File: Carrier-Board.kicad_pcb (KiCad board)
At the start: 2 copper layers, 92 x 96 mm, 5 parts, among them J1 CONN_3-6318491-6, J2 SI-51009-F, U1 MSATA-Socket, X1 PC104_PLUS

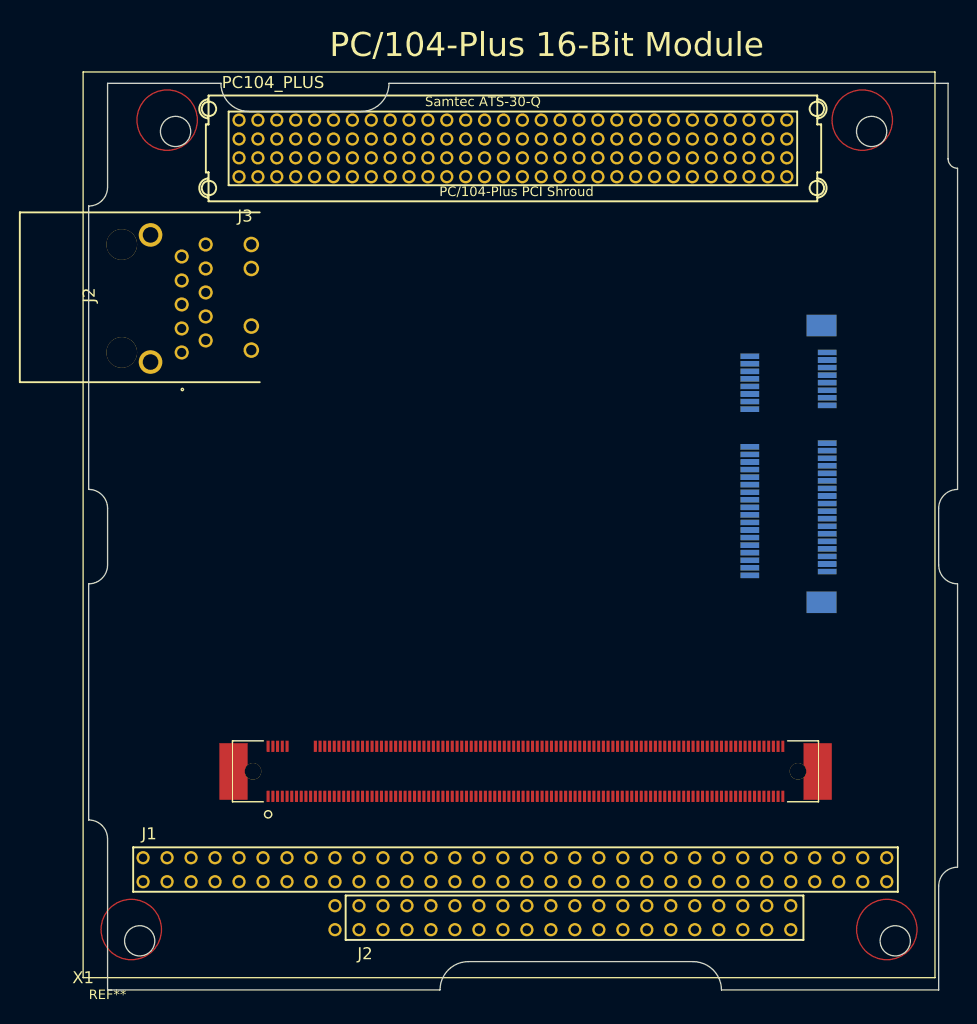
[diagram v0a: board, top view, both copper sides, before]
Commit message: Remove junk from pc104
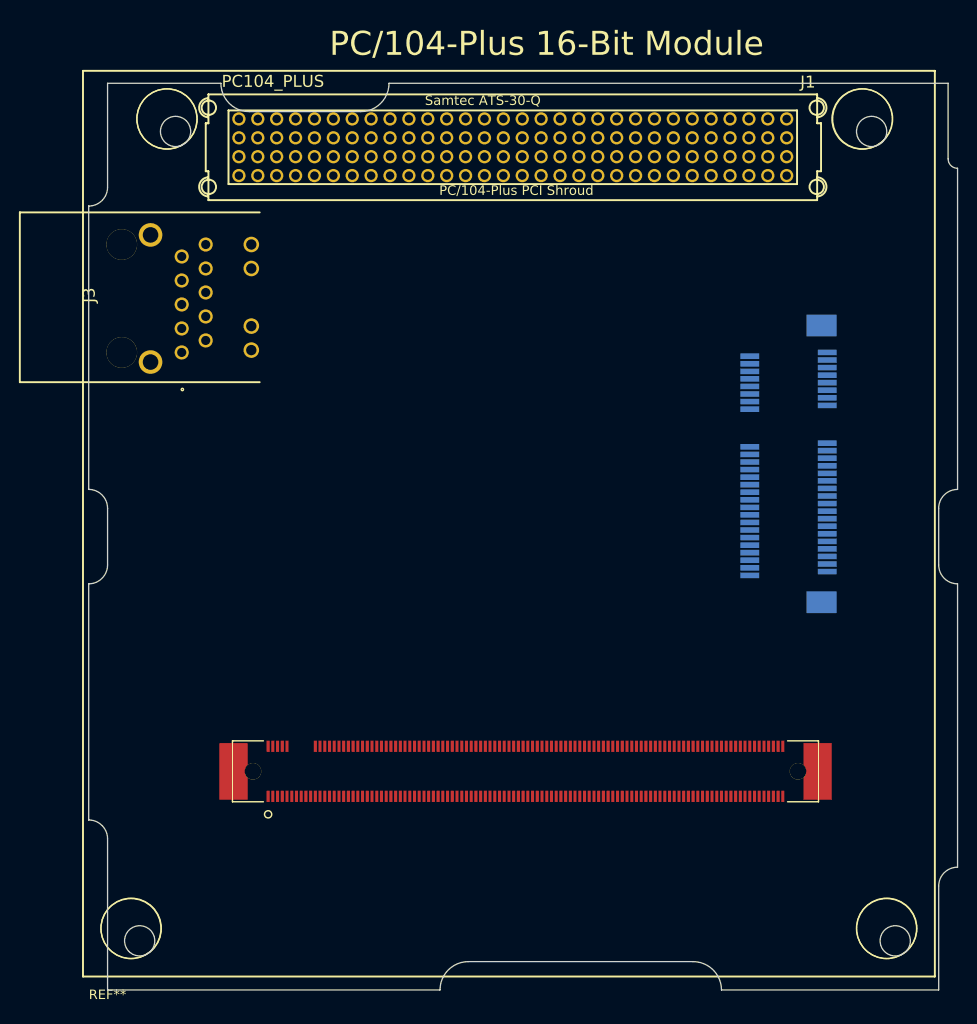
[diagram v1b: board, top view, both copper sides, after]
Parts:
- removed X1: PC104_PLUS, Carrier-Board:con-pc104-PC104-PLUS
- added J1: PC104_PLUS, Carrier-Board:pc104_silk, F.Cu at (54.4, 126.1)
- J2: renamed from J1; value CONN_3-6318491-6 -> PC104_PLUS
- renumbered J2 to J3
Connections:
- J2 pad 1: Net-(J1-Pad1) -> (no net)
- J2 pad 10: Net-(J1-Pad10) -> (no net)
- J2 pad 100: Net-(J1-Pad100) -> (no net)
- J2 pad 101: Net-(J1-Pad101) -> (no net)
- J2 pad 102: Net-(J1-Pad102) -> (no net)
- J2 pad 103: Net-(J1-Pad103) -> (no net)
- J2 pad 104: Net-(J1-Pad104) -> (no net)
- J2 pad 105: Net-(J1-Pad105) -> (no net)
- J2 pad 106: Net-(J1-Pad106) -> (no net)
- J2 pad 107: Net-(J1-Pad107) -> (no net)
- J2 pad 108: Net-(J1-Pad108) -> (no net)
- J2 pad 109: Net-(J1-Pad109) -> (no net)
- J2 pad 11: Net-(J1-Pad11) -> (no net)
- J2 pad 110: Net-(J1-Pad110) -> (no net)
- J2 pad 111: Net-(J1-Pad111) -> (no net)
- J2 pad 112: Net-(J1-Pad112) -> (no net)
- J2 pad 113: Net-(J1-Pad113) -> (no net)
- J2 pad 114: Net-(J1-Pad114) -> (no net)
- J2 pad 115: Net-(J1-Pad115) -> (no net)
- J2 pad 12: Net-(J1-Pad12) -> (no net)
- J2 pad 121: Net-(J1-Pad121) -> (no net)
- J2 pad 122: Net-(J1-Pad122) -> (no net)
- J2 pad 123: Net-(J1-Pad123) -> (no net)
- J2 pad 124: Net-(J1-Pad124) -> (no net)
- J2 pad 125: Net-(J1-Pad125) -> (no net)
- J2 pad 126: Net-(J1-Pad126) -> (no net)
- J2 pad 127: Net-(J1-Pad127) -> (no net)
- J2 pad 128: Net-(J1-Pad128) -> (no net)
- J2 pad 129: Net-(J1-Pad129) -> (no net)
- J2 pad 13: Net-(J1-Pad13) -> (no net)
- J2 pad 130: Net-(J1-Pad130) -> (no net)
- J2 pad 131: Net-(J1-Pad131) -> (no net)
- J2 pad 132: Net-(J1-Pad132) -> (no net)
- J2 pad 133: Net-(J1-Pad133) -> (no net)
- J2 pad 134: Net-(J1-Pad134) -> (no net)
- J2 pad 135: Net-(J1-Pad135) -> (no net)
- J2 pad 136: Net-(J1-Pad136) -> (no net)
- J2 pad 137: Net-(J1-Pad137) -> (no net)
- J2 pad 138: Net-(J1-Pad138) -> (no net)
- J2 pad 139: Net-(J1-Pad139) -> (no net)
- J2 pad 14: Net-(J1-Pad14) -> (no net)
- J2 pad 140: Net-(J1-Pad140) -> (no net)
- J2 pad 141: Net-(J1-Pad141) -> (no net)
- J2 pad 142: Net-(J1-Pad142) -> (no net)
- J2 pad 143: Net-(J1-Pad143) -> (no net)
- J2 pad 144: Net-(J1-Pad144) -> (no net)
- J2 pad 145: Net-(J1-Pad145) -> (no net)
- J2 pad 146: Net-(J1-Pad146) -> (no net)
- J2 pad 147: Net-(J1-Pad147) -> (no net)
- J2 pad 148: Net-(J1-Pad148) -> (no net)
- J2 pad 149: Net-(J1-Pad149) -> (no net)
- J2 pad 15: Net-(J1-Pad15) -> (no net)
- J2 pad 150: Net-(J1-Pad150) -> (no net)
- J2 pad 151: Net-(J1-Pad151) -> (no net)
- J2 pad 152: Net-(J1-Pad152) -> (no net)
- J2 pad 153: Net-(J1-Pad153) -> (no net)
- J2 pad 154: Net-(J1-Pad154) -> (no net)
- J2 pad 155: Net-(J1-Pad155) -> (no net)
- J2 pad 156: Net-(J1-Pad156) -> (no net)
- J2 pad 157: Net-(J1-Pad157) -> (no net)
- J2 pad 158: Net-(J1-Pad158) -> (no net)
- J2 pad 159: Net-(J1-Pad159) -> (no net)
- J2 pad 16: Net-(J1-Pad16) -> (no net)
- J2 pad 160: Net-(J1-Pad160) -> (no net)
- J2 pad 161: Net-(J1-Pad161) -> (no net)
- J2 pad 162: Net-(J1-Pad162) -> (no net)
- J2 pad 163: Net-(J1-Pad163) -> (no net)
- J2 pad 164: Net-(J1-Pad164) -> (no net)
- J2 pad 165: Net-(J1-Pad165) -> (no net)
- J2 pad 166: Net-(J1-Pad166) -> (no net)
- J2 pad 167: Net-(J1-Pad167) -> (no net)
- J2 pad 168: Net-(J1-Pad168) -> (no net)
- J2 pad 169: Net-(J1-Pad169) -> (no net)
- J2 pad 17: Net-(J1-Pad17) -> (no net)
- J2 pad 170: Net-(J1-Pad170) -> (no net)
- J2 pad 171: Net-(J1-Pad171) -> (no net)
- J2 pad 172: Net-(J1-Pad172) -> (no net)
- J2 pad 173: Net-(J1-Pad173) -> (no net)
- J2 pad 174: Net-(J1-Pad174) -> (no net)
- J2 pad 175: Net-(J1-Pad175) -> (no net)
- J2 pad 176: Net-(J1-Pad176) -> (no net)
- J2 pad 177: Net-(J1-Pad177) -> (no net)
- J2 pad 178: Net-(J1-Pad178) -> (no net)
- J2 pad 179: Net-(J1-Pad179) -> (no net)
- J2 pad 18: Net-(J1-Pad18) -> (no net)
- J2 pad 180: Net-(J1-Pad180) -> (no net)
- J2 pad 181: Net-(J1-Pad181) -> (no net)
- J2 pad 182: Net-(J1-Pad182) -> (no net)
- J2 pad 183: Net-(J1-Pad183) -> (no net)
- J2 pad 184: Net-(J1-Pad184) -> (no net)
- J2 pad 185: Net-(J1-Pad185) -> (no net)
- J2 pad 186: Net-(J1-Pad186) -> (no net)
- J2 pad 187: Net-(J1-Pad187) -> (no net)
- J2 pad 188: Net-(J1-Pad188) -> (no net)
- J2 pad 189: Net-(J1-Pad189) -> (no net)
- J2 pad 19: Net-(J1-Pad19) -> (no net)
- J2 pad 190: Net-(J1-Pad190) -> (no net)
- J2 pad 191: Net-(J1-Pad191) -> (no net)
- J2 pad 192: Net-(J1-Pad192) -> (no net)
- J2 pad 193: Net-(J1-Pad193) -> (no net)
- J2 pad 194: Net-(J1-Pad194) -> (no net)
- J2 pad 195: Net-(J1-Pad195) -> (no net)
- J2 pad 196: Net-(J1-Pad196) -> (no net)
- J2 pad 197: Net-(J1-Pad197) -> (no net)
- J2 pad 198: Net-(J1-Pad198) -> (no net)
- J2 pad 199: Net-(J1-Pad199) -> (no net)
- J2 pad 2: Net-(J1-Pad2) -> (no net)
- J2 pad 20: Net-(J1-Pad20) -> (no net)
- J2 pad 200: Net-(J1-Pad200) -> (no net)
- J2 pad 201: Net-(J1-Pad201) -> (no net)
- J2 pad 202: Net-(J1-Pad202) -> (no net)
- J2 pad 203: Net-(J1-Pad203) -> (no net)
- J2 pad 204: Net-(J1-Pad204) -> (no net)
- J2 pad 205: Net-(J1-Pad205) -> (no net)
- J2 pad 206: Net-(J1-Pad206) -> (no net)
- J2 pad 207: Net-(J1-Pad207) -> (no net)
- J2 pad 208: Net-(J1-Pad208) -> (no net)
- J2 pad 209: Net-(J1-Pad209) -> (no net)
- J2 pad 21: Net-(J1-Pad21) -> (no net)
- J2 pad 210: Net-(J1-Pad210) -> (no net)
- J2 pad 211: Net-(J1-Pad211) -> (no net)
- J2 pad 212: Net-(J1-Pad212) -> (no net)
- J2 pad 213: Net-(J1-Pad213) -> (no net)
- J2 pad 214: Net-(J1-Pad214) -> (no net)
- J2 pad 215: Net-(J1-Pad215) -> (no net)
- J2 pad 216: Net-(J1-Pad216) -> (no net)
- J2 pad 217: Net-(J1-Pad217) -> (no net)
- J2 pad 218: Net-(J1-Pad218) -> (no net)
- J2 pad 219: Net-(J1-Pad219) -> (no net)
- J2 pad 22: Net-(J1-Pad22) -> (no net)
- J2 pad 220: Net-(J1-Pad220) -> (no net)
- J2 pad 23: Net-(J1-Pad23) -> (no net)
- J2 pad 24: Net-(J1-Pad24) -> (no net)
- J2 pad 25: Net-(J1-Pad25) -> (no net)
- J2 pad 26: Net-(J1-Pad26) -> (no net)
- J2 pad 27: Net-(J1-Pad27) -> (no net)
- J2 pad 28: Net-(J1-Pad28) -> (no net)
- J2 pad 29: Net-(J1-Pad29) -> (no net)
- J2 pad 3: Net-(J1-Pad3) -> (no net)
- J2 pad 30: Net-(J1-Pad30) -> (no net)
- J2 pad 31: Net-(J1-Pad31) -> (no net)
- J2 pad 32: Net-(J1-Pad32) -> (no net)
- J2 pad 33: Net-(J1-Pad33) -> (no net)
- J2 pad 34: Net-(J1-Pad34) -> (no net)
- J2 pad 35: Net-(J1-Pad35) -> (no net)
- J2 pad 36: Net-(J1-Pad36) -> (no net)
- J2 pad 37: Net-(J1-Pad37) -> (no net)
- J2 pad 38: Net-(J1-Pad38) -> (no net)
- J2 pad 39: Net-(J1-Pad39) -> (no net)
- J2 pad 4: Net-(J1-Pad4) -> (no net)
- J2 pad 40: Net-(J1-Pad40) -> (no net)
- J2 pad 41: Net-(J1-Pad41) -> (no net)
- J2 pad 42: Net-(J1-Pad42) -> (no net)
- J2 pad 43: Net-(J1-Pad43) -> (no net)
- J2 pad 44: Net-(J1-Pad44) -> (no net)
- J2 pad 45: Net-(J1-Pad45) -> (no net)
- J2 pad 46: Net-(J1-Pad46) -> (no net)
- J2 pad 47: Net-(J1-Pad47) -> (no net)
- J2 pad 48: Net-(J1-Pad48) -> (no net)
- J2 pad 49: Net-(J1-Pad49) -> (no net)
- J2 pad 5: Net-(J1-Pad5) -> (no net)
- J2 pad 50: Net-(J1-Pad50) -> (no net)
- J2 pad 51: Net-(J1-Pad51) -> (no net)
- J2 pad 52: Net-(J1-Pad52) -> (no net)
- J2 pad 53: Net-(J1-Pad53) -> (no net)
- J2 pad 54: Net-(J1-Pad54) -> (no net)
- J2 pad 55: Net-(J1-Pad55) -> (no net)
- J2 pad 56: Net-(J1-Pad56) -> (no net)
- J2 pad 57: Net-(J1-Pad57) -> (no net)
- J2 pad 58: Net-(J1-Pad58) -> (no net)
- J2 pad 59: Net-(J1-Pad59) -> (no net)
- J2 pad 6: Net-(J1-Pad6) -> (no net)
- J2 pad 60: Net-(J1-Pad60) -> (no net)
- J2 pad 61: Net-(J1-Pad61) -> (no net)
- J2 pad 62: Net-(J1-Pad62) -> (no net)
- J2 pad 63: Net-(J1-Pad63) -> (no net)
- J2 pad 64: Net-(J1-Pad64) -> (no net)
- J2 pad 65: Net-(J1-Pad65) -> (no net)
- J2 pad 66: Net-(J1-Pad66) -> (no net)
- J2 pad 67: Net-(J1-Pad67) -> (no net)
- J2 pad 68: Net-(J1-Pad68) -> (no net)
- J2 pad 69: Net-(J1-Pad69) -> (no net)
- J2 pad 7: Net-(J1-Pad7) -> (no net)
- J2 pad 70: Net-(J1-Pad70) -> (no net)
- J2 pad 71: Net-(J1-Pad71) -> (no net)
- J2 pad 72: Net-(J1-Pad72) -> (no net)
- J2 pad 73: Net-(J1-Pad73) -> (no net)
- J2 pad 74: Net-(J1-Pad74) -> (no net)
- J2 pad 75: Net-(J1-Pad75) -> (no net)
- J2 pad 76: Net-(J1-Pad76) -> (no net)
- J2 pad 77: Net-(J1-Pad77) -> (no net)
- J2 pad 78: Net-(J1-Pad78) -> (no net)
- J2 pad 79: Net-(J1-Pad79) -> (no net)
- J2 pad 8: Net-(J1-Pad8) -> (no net)
- J2 pad 80: Net-(J1-Pad80) -> (no net)
- J2 pad 81: Net-(J1-Pad81) -> (no net)
- J2 pad 82: Net-(J1-Pad82) -> (no net)
- J2 pad 83: Net-(J1-Pad83) -> (no net)
- J2 pad 84: Net-(J1-Pad84) -> (no net)
- J2 pad 85: Net-(J1-Pad85) -> (no net)
- J2 pad 86: Net-(J1-Pad86) -> (no net)
- J2 pad 87: Net-(J1-Pad87) -> (no net)
- J2 pad 88: Net-(J1-Pad88) -> (no net)
- J2 pad 89: Net-(J1-Pad89) -> (no net)
- J2 pad 9: Net-(J1-Pad9) -> (no net)
- J2 pad 90: Net-(J1-Pad90) -> (no net)
- J2 pad 91: Net-(J1-Pad91) -> (no net)
- J2 pad 92: Net-(J1-Pad92) -> (no net)
- J2 pad 93: Net-(J1-Pad93) -> (no net)
- J2 pad 94: Net-(J1-Pad94) -> (no net)
- J2 pad 95: Net-(J1-Pad95) -> (no net)
- J2 pad 96: Net-(J1-Pad96) -> (no net)
- J2 pad 97: Net-(J1-Pad97) -> (no net)
- J2 pad 98: Net-(J1-Pad98) -> (no net)
- J2 pad 99: Net-(J1-Pad99) -> (no net)
- J3 pad 1: Net-(J2-Pad1) -> (no net)
- J3 pad 10: Net-(J2-Pad10) -> (no net)
- J3 pad 2: Net-(J2-Pad2) -> (no net)
- J3 pad 3: Net-(J2-Pad3) -> (no net)
- J3 pad 4: Net-(J2-Pad4) -> (no net)
- J3 pad 5: Net-(J2-Pad5) -> (no net)
- J3 pad 6: Net-(J2-Pad6) -> (no net)
- J3 pad 7: Net-(J2-Pad7) -> (no net)
- J3 pad 8: Net-(J2-Pad8) -> (no net)
- J3 pad 9: Net-(J2-Pad9) -> (no net)
- U1 pad 1: Net-(U1-Pad1) -> (no net)
- U1 pad 10: Net-(U1-Pad10) -> (no net)
- U1 pad 11: Net-(U1-Pad11) -> (no net)
- U1 pad 12: Net-(U1-Pad12) -> (no net)
- U1 pad 13: Net-(U1-Pad13) -> (no net)
- U1 pad 14: Net-(U1-Pad14) -> (no net)
- U1 pad 15: Net-(U1-Pad15) -> (no net)
- U1 pad 16: Net-(U1-Pad16) -> (no net)
- U1 pad 17: Net-(U1-Pad17) -> (no net)
- U1 pad 18: Net-(U1-Pad18) -> (no net)
- U1 pad 19: Net-(U1-Pad19) -> (no net)
- U1 pad 2: Net-(U1-Pad2) -> (no net)
- U1 pad 20: Net-(U1-Pad20) -> (no net)
- U1 pad 21: Net-(U1-Pad21) -> (no net)
- U1 pad 22: Net-(U1-Pad22) -> (no net)
- U1 pad 23: Net-(U1-Pad23) -> (no net)
- U1 pad 24: Net-(U1-Pad24) -> (no net)
- U1 pad 25: Net-(U1-Pad25) -> (no net)
- U1 pad 26: Net-(U1-Pad26) -> (no net)
- U1 pad 27: Net-(U1-Pad27) -> (no net)
- U1 pad 28: Net-(U1-Pad28) -> (no net)
- U1 pad 29: Net-(U1-Pad29) -> (no net)
- U1 pad 3: Net-(U1-Pad3) -> (no net)
- U1 pad 30: Net-(U1-Pad30) -> (no net)
- U1 pad 31: Net-(U1-Pad31) -> (no net)
- U1 pad 32: Net-(U1-Pad32) -> (no net)
- U1 pad 33: Net-(U1-Pad33) -> (no net)
- U1 pad 34: Net-(U1-Pad34) -> (no net)
- U1 pad 35: Net-(U1-Pad35) -> (no net)
- U1 pad 36: Net-(U1-Pad36) -> (no net)
- U1 pad 37: Net-(U1-Pad37) -> (no net)
- U1 pad 38: Net-(U1-Pad38) -> (no net)
- U1 pad 39: Net-(U1-Pad39) -> (no net)
- U1 pad 4: Net-(U1-Pad4) -> (no net)
- U1 pad 40: Net-(U1-Pad40) -> (no net)
- U1 pad 41: Net-(U1-Pad41) -> (no net)
- U1 pad 42: Net-(U1-Pad42) -> (no net)
- U1 pad 43: Net-(U1-Pad43) -> (no net)
- U1 pad 44: Net-(U1-Pad44) -> (no net)
- U1 pad 45: Net-(U1-Pad45) -> (no net)
- U1 pad 46: Net-(U1-Pad46) -> (no net)
- U1 pad 47: Net-(U1-Pad47) -> (no net)
- U1 pad 48: Net-(U1-Pad48) -> (no net)
- U1 pad 49: Net-(U1-Pad49) -> (no net)
- U1 pad 5: Net-(U1-Pad5) -> (no net)
- U1 pad 50: Net-(U1-Pad50) -> (no net)
- U1 pad 51: Net-(U1-Pad51) -> (no net)
- U1 pad 52: Net-(U1-Pad52) -> (no net)
- U1 pad 6: Net-(U1-Pad6) -> (no net)
- U1 pad 7: Net-(U1-Pad7) -> (no net)
- U1 pad 8: Net-(U1-Pad8) -> (no net)
- U1 pad 9: Net-(U1-Pad9) -> (no net)

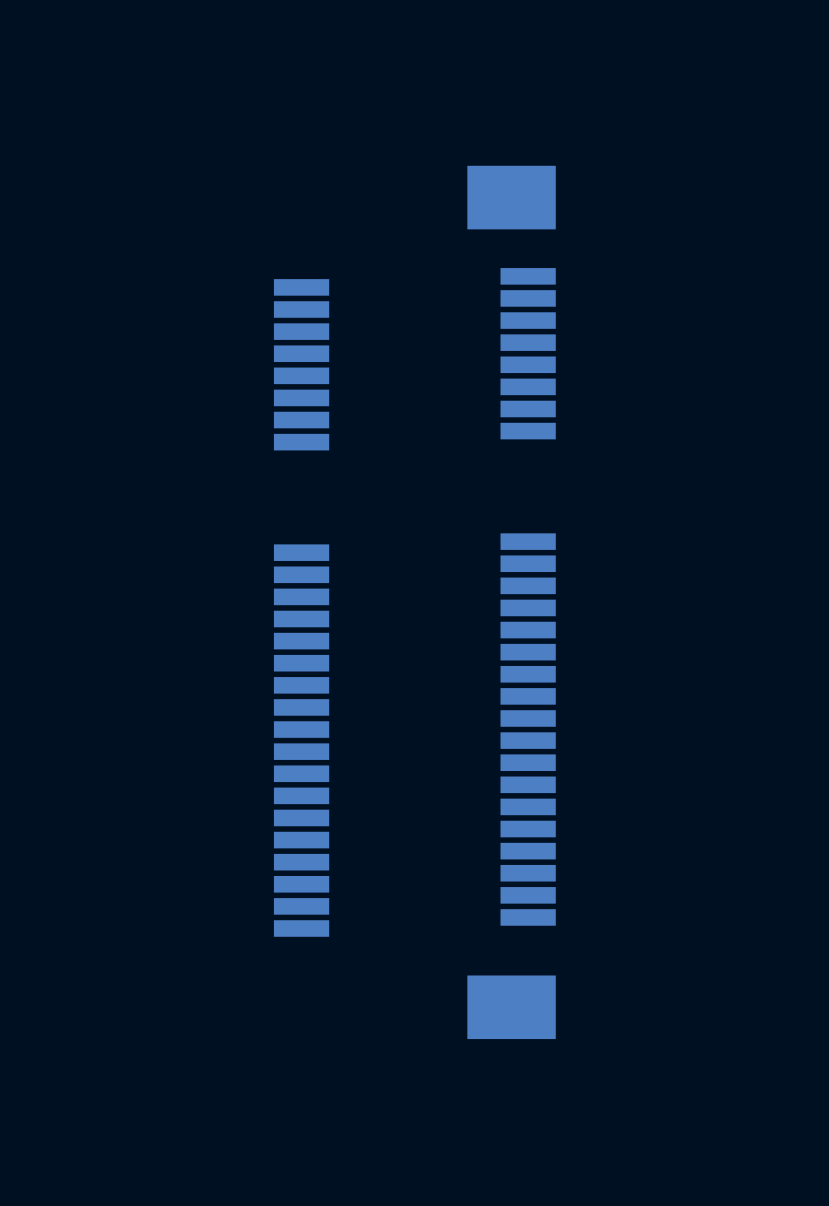
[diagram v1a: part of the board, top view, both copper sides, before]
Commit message: 'kidz
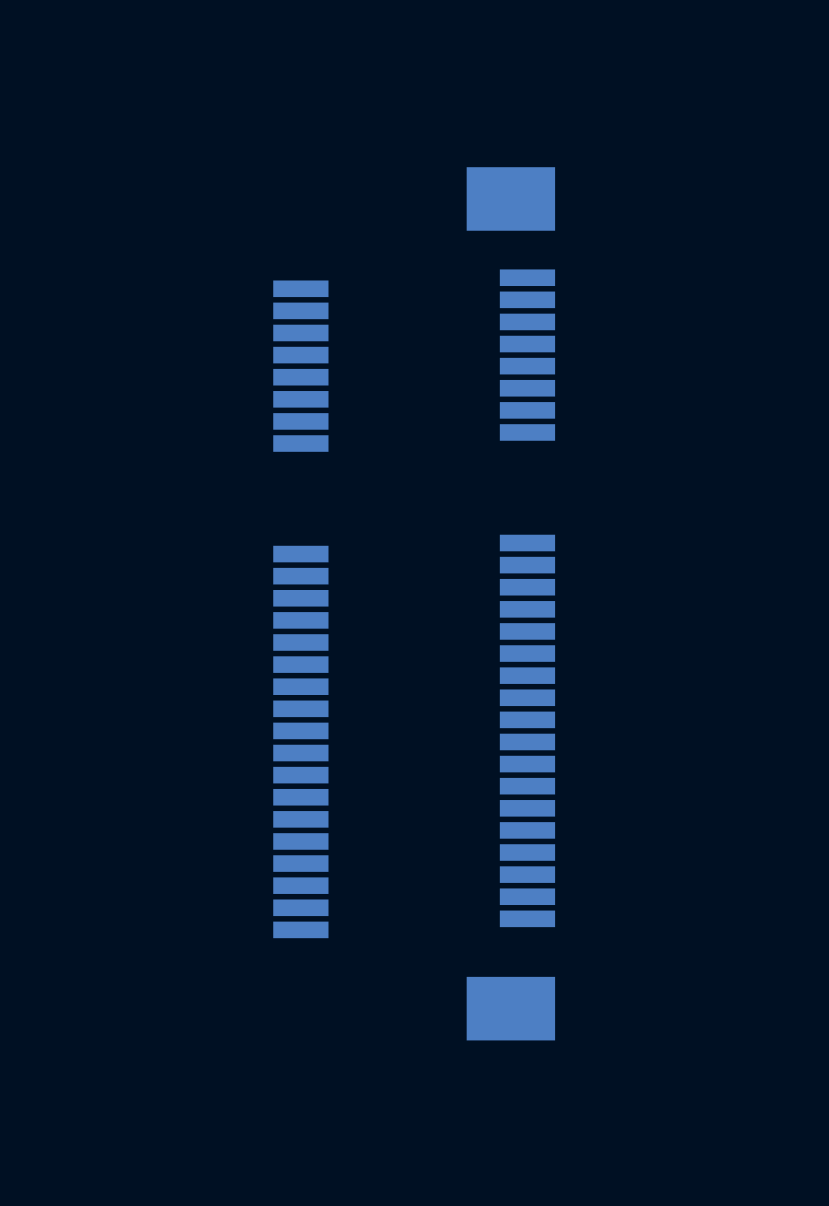
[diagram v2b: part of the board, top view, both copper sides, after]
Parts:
- moved U1 0.06 mm to (129.1, 59.4)
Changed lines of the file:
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@@
     (links 116)
     (no_connects 116)
-    (area 0 0 0 0)
+    (area 41.471239 29.878679 157.492041 139.003381)
     (thickness 1.6)
     (drawings 0)
@@
   )
   (module Carrier-Board:msata-socket (layer B.Cu)
-    (at 129.1 59.3 270)
+    (at 129.075 59.35 270)
     (tags "mpci, pci, pci express")
     (fp_text reference U1 (at 30.45 -2.45 540) (layer B.SilkS) hide
